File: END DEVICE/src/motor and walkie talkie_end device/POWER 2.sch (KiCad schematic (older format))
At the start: 31 parts, among them IC4 TPS55340RTER, SW6 SW_SPDT, U7 LM117_TO39, U8 LM741

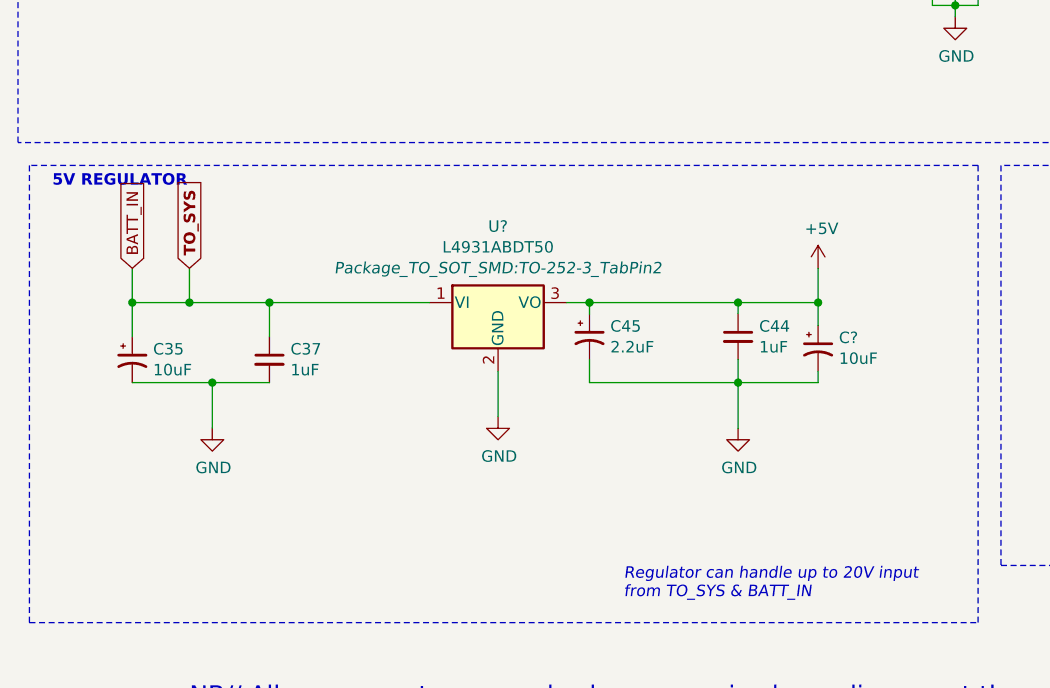
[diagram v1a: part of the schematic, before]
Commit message: third commit:very minor changes
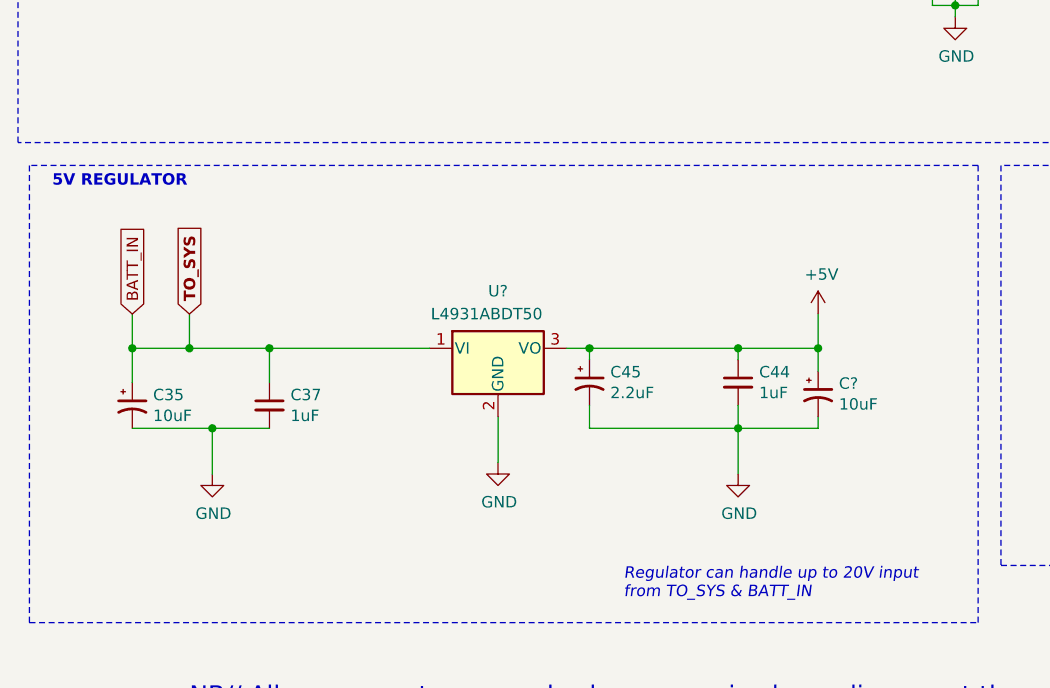
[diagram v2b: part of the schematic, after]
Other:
- moved on the sheet: C35, C37, C44, C45, C?, U?
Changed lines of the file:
@@
 Text Notes 750  4850 0    50   ~ 10
 5V REGULATOR
-Connection ~ 4100 5350
-Wire Wire Line
-	4100 5350 4100 5200
+Connection ~ 4100 5550
+Wire Wire Line
+	4100 5550 4100 5400
 $Comp
 L power:+5V #PWR0173
 U 1 1 61EC74E6
-P 4100 5200
-F 0 "#PWR0173" H 4100 5050 50  0001 C CNN
-F 1 "+5V" H 4115 5373 50  0000 C CNN
-F 2 "" H 4100 5200 50  0001 C CNN
-F 3 "" H 4100 5200 50  0001 C CNN
-	1    4100 5200
-	1    0    0    -1
-$EndComp
-Wire Wire Line
-	1700 5350 1350 5350
-Connection ~ 1700 5350
-Wire Wire Line
-	1700 5500 1700 5350
-Wire Wire Line
-	1100 5500 1100 5350
-Wire Wire Line
-	1450 5700 1700 5700
-Connection ~ 1450 5700
-Wire Wire Line
-	1450 5700 1100 5700
-Wire Wire Line
-	1450 5900 1450 5700
+P 4100 5400
+F 0 "#PWR0173" H 4100 5250 50  0001 C CNN
+F 1 "+5V" H 4115 5573 50  0000 C CNN
+F 2 "" H 4100 5400 50  0001 C CNN
+F 3 "" H 4100 5400 50  0001 C CNN
+	1    4100 5400
+	1    0    0    -1
+$EndComp
+Wire Wire Line
+	1700 5550 1350 5550
+Connection ~ 1700 5550
+Wire Wire Line
+	1700 5700 1700 5550
+Wire Wire Line
+	1100 5700 1100 5550
+Wire Wire Line
+	1450 5900 1700 5900
+Connection ~ 1450 5900
+Wire Wire Line
+	1450 5900 1100 5900
+Wire Wire Line
+	1450 6100 1450 5900
 $Comp
 L power:GND #PWR0174
 U 1 1 61EAEFFC
-P 1450 5900
-F 0 "#PWR0174" H 1450 5650 50  0001 C CNN
-F 1 "GND" H 1455 5727 50  0000 C CNN
-F 2 "" H 1450 5900 50  0001 C CNN
-F 3 "" H 1450 5900 50  0001 C CNN
-	1    1450 5900
-	1    0    0    -1
-$EndComp
-Connection ~ 3750 5700
-Wire Wire Line
-	3750 5900 3750 5700
+P 1450 6100
+F 0 "#PWR0174" H 1450 5850 50  0001 C CNN
+F 1 "GND" H 1455 5927 50  0000 C CNN
+F 2 "" H 1450 6100 50  0001 C CNN
+F 3 "" H 1450 6100 50  0001 C CNN
+	1    1450 6100
+	1    0    0    -1
+$EndComp
+Connection ~ 3750 5900
+Wire Wire Line
+	3750 6100 3750 5900
 $Comp
 L power:GND #PWR0175
 U 1 1 61EA92A1
-P 3750 5900
-F 0 "#PWR0175" H 3750 5650 50  0001 C CNN
-F 1 "GND" H 3755 5727 50  0000 C CNN
-F 2 "" H 3750 5900 50  0001 C CNN
-F 3 "" H 3750 5900 50  0001 C CNN
-	1    3750 5900
+P 3750 6100
+F 0 "#PWR0175" H 3750 5850 50  0001 C CNN
+F 1 "GND" H 3755 5927 50  0000 C CNN
+F 2 "" H 3750 6100 50  0001 C CNN
+F 3 "" H 3750 6100 50  0001 C CNN
+	1    3750 6100
 	1    0    0    -1
 $EndComp
@@
 L power:GND #PWR0176
 U 1 1 61EA7291
-P 2700 5850
-F 0 "#PWR0176" H 2700 5600 50  0001 C CNN
-F 1 "GND" H 2705 5677 50  0000 C CNN
-F 2 "" H 2700 5850 50  0001 C CNN
-F 3 "" H 2700 5850 50  0001 C CNN
-	1    2700 5850
-	1    0    0    -1
-$EndComp
-Wire Wire Line
-	4100 5350 4100 5450
-Wire Wire Line
-	3750 5350 3750 5400
+P 2700 6050
+F 0 "#PWR0176" H 2700 5800 50  0001 C CNN
+F 1 "GND" H 2705 5877 50  0000 C CNN
+F 2 "" H 2700 6050 50  0001 C CNN
+F 3 "" H 2700 6050 50  0001 C CNN
+	1    2700 6050
+	1    0    0    -1
+$EndComp
+Wire Wire Line
+	4100 5550 4100 5650
+Wire Wire Line
+	3750 5550 3750 5600
 $Comp
 L Device:CP1_Small C45
 U 1 1 61E99AAF
-P 3100 5500
-F 0 "C45" H 3191 5546 50  0000 L CNN
-F 1 "2.2uF" H 3191 5455 50  0000 L CNN
-F 2 "" H 3100 5500 50  0001 C CNN
-F 3 "~" H 3100 5500 50  0001 C CNN
-	1    3100 5500
+P 3100 5700
+F 0 "C45" H 3191 5746 50  0000 L CNN
+F 1 "2.2uF" H 3191 5655 50  0000 L CNN
+F 2 "" H 3100 5700 50  0001 C CNN
+F 3 "~" H 3100 5700 50  0001 C CNN
+	1    3100 5700
 	1    0    0    -1
 $EndComp
@@
 L Device:C_Small C37
 U 1 1 61E9952A
-P 1700 5600
-F 0 "C37" H 1792 5646 50  0000 L CNN
-F 1 "1uF" H 1792 5555 50  0000 L CNN
-F 2 "" H 1700 5600 50  0001 C CNN
-F 3 "~" H 1700 5600 50  0001 C CNN
-	1    1700 5600
+P 1700 5800
+F 0 "C37" H 1792 5846 50  0000 L CNN
+F 1 "1uF" H 1792 5755 50  0000 L CNN
+F 2 "" H 1700 5800 50  0001 C CNN
+F 3 "~" H 1700 5800 50  0001 C CNN
+	1    1700 5800
 	1    0    0    -1
 $EndComp
@@
 L Device:CP1_Small C35
 U 1 1 61E98783
-P 1100 5600
-F 0 "C35" H 1191 5646 50  0000 L CNN
-F 1 "10uF" H 1191 5555 50  0000 L CNN
-F 2 "" H 1100 5600 50  0001 C CNN
-F 3 "~" H 1100 5600 50  0001 C CNN
-	1    1100 5600
+P 1100 5800
+F 0 "C35" H 1191 5846 50  0000 L CNN
+F 1 "10uF" H 1191 5755 50  0000 L CNN
+F 2 "" H 1100 5800 50  0001 C CNN
+F 3 "~" H 1100 5800 50  0001 C CNN
+	1    1100 5800
 	1    0    0    -1
 $EndComp
@@
 Wire Wire Line
 	1700 950  1700 1100
-Text GLabel 1100 5200 1    50   Input ~ 0
+Text GLabel 1100 5400 1    50   Input ~ 0
 BATT_IN
 Wire Wire Line
-	1100 5200 1100 5350
-Connection ~ 1100 5350
+	1100 5400 1100 5550
+Connection ~ 1100 5550
 Text GLabel 1800 950  1    50   Input ~ 0
 BATT_IN
@@
 L remote_devices:L4931ABDT50 U?
 U 1 1 62291361
-P 2700 5350
-F 0 "U?" H 2700 5683 50  0000 C CNN
-F 1 "L4931ABDT50" H 2700 5592 50  0000 C CNN
-F 2 "Package_TO_SOT_SMD:TO-252-3_TabPin2" H 2700 5501 50  0000 C CIN
-F 3 "" H 2700 5300 50  0001 C CNN
-	1    2700 5350
-	1    0    0    -1
-$EndComp
-Wire Wire Line
-	1700 5350 2400 5350
-Wire Wire Line
-	3000 5350 3100 5350
-Wire Wire Line
-	2700 5650 2700 5850
-Text GLabel 1350 5200 1    50   Input ~ 10
+P 2700 5550
+F 0 "U?" H 2700 5800 50  0000 C CNN
+F 1 "L4931ABDT50" H 2650 5700 50  0000 C CNN
+F 2 "Package_TO_SOT_SMD:TO-252-3_TabPin2" H 2700 5701 50  0001 C CIN
+F 3 "" H 2700 5500 50  0001 C CNN
+	1    2700 5550
+	1    0    0    -1
+$EndComp
+Wire Wire Line
+	1700 5550 2400 5550
+Wire Wire Line
+	3000 5550 3100 5550
+Wire Wire Line
+	2700 5850 2700 6050
+Text GLabel 1350 5400 1    50   Input ~ 10
 TO_SYS
 Wire Wire Line
-	1350 5200 1350 5350
-Connection ~ 1350 5350
-Wire Wire Line
-	1350 5350 1100 5350
+	1350 5400 1350 5550
+Connection ~ 1350 5550
+Wire Wire Line
+	1350 5550 1100 5550
 Text Notes 3250 6650 0    50   Italic 0
 Regulator can handle up to 20V input \nfrom TO_SYS & BATT_IN
 Wire Wire Line
-	3100 5400 3100 5350
-Connection ~ 3100 5350
-Wire Wire Line
-	3100 5600 3100 5700
+	3100 5600 3100 5550
+Connection ~ 3100 5550
+Wire Wire Line
+	3100 5800 3100 5900
 $Comp
 L Device:CP1_Small C?
 U 1 1 622D1115
-P 4100 5550
-F 0 "C?" H 4191 5596 50  0000 L CNN
-F 1 "10uF" H 4191 5505 50  0000 L CNN
-F 2 "" H 4100 5550 50  0001 C CNN
-F 3 "~" H 4100 5550 50  0001 C CNN
-	1    4100 5550
-	1    0    0    -1
-$EndComp
-Wire Wire Line
-	4100 5700 4100 5650
-Wire Wire Line
-	3750 5700 4100 5700
+P 4100 5750
+F 0 "C?" H 4191 5796 50  0000 L CNN
+F 1 "10uF" H 4191 5705 50  0000 L CNN
+F 2 "" H 4100 5750 50  0001 C CNN
+F 3 "~" H 4100 5750 50  0001 C CNN
+	1    4100 5750
+	1    0    0    -1
+$EndComp
+Wire Wire Line
+	4100 5900 4100 5850
+Wire Wire Line
+	3750 5900 4100 5900
 $Comp
 L Device:C_Small C44
 U 1 1 61E99AB9
-P 3750 5500
-F 0 "C44" H 3842 5546 50  0000 L CNN
-F 1 "1uF" H 3842 5455 50  0000 L CNN
-F 2 "" H 3750 5500 50  0001 C CNN
-F 3 "~" H 3750 5500 50  0001 C CNN
-	1    3750 5500
-	1    0    0    -1
-$EndComp
-Wire Wire Line
-	3750 5600 3750 5700
-Connection ~ 3750 5350
-Wire Wire Line
-	3750 5350 4100 5350
-Wire Wire Line
-	3100 5350 3750 5350
-Wire Wire Line
-	3100 5700 3750 5700
+P 3750 5700
+F 0 "C44" H 3842 5746 50  0000 L CNN
+F 1 "1uF" H 3842 5655 50  0000 L CNN
+F 2 "" H 3750 5700 50  0001 C CNN
+F 3 "~" H 3750 5700 50  0001 C CNN
+	1    3750 5700
+	1    0    0    -1
+$EndComp
+Wire Wire Line
+	3750 5800 3750 5900
+Connection ~ 3750 5550
+Wire Wire Line
+	3750 5550 4100 5550
+Wire Wire Line
+	3100 5550 3750 5550
+Wire Wire Line
+	3100 5900 3750 5900
 Text Notes 1350 7250 0    79   ~ 0
 NB// All components can work when power is pluggedin except the\n         DC-Motor. The motor only works when the battery is connected
